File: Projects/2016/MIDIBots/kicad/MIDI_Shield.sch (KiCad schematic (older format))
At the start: 45 parts, among them IC1 PC900V, K1 SERVO_1, K2 SERVO_2, K3 SERVO_3, P1 MIDI_IN, P2 MIDI_THRU, P3 PWR_IN, P4 MIDI_IN, P5 MIDI_THRU, P6 D6_PWM, P7 MIDI_RX_EN, P8 STEPPER, P9 D12, Q1 F12N10L, Q2 F12N10L, SW1 RESET, SW2 DIPS_04, SW3 SELF_TEST, U1 74HC14

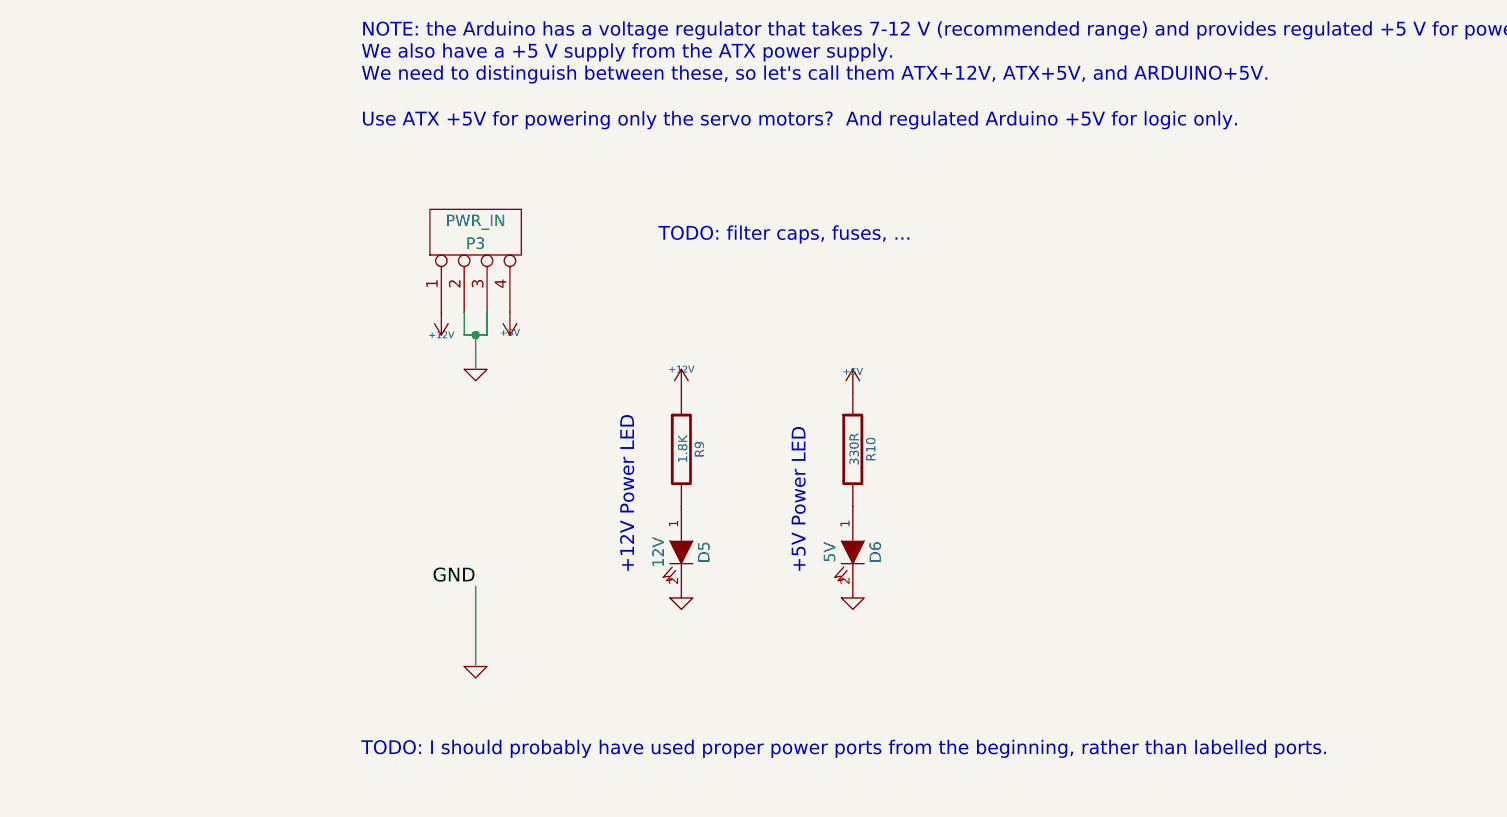
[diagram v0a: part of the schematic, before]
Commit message: Latest schematic and PCB design from work, plus extra libs we might need
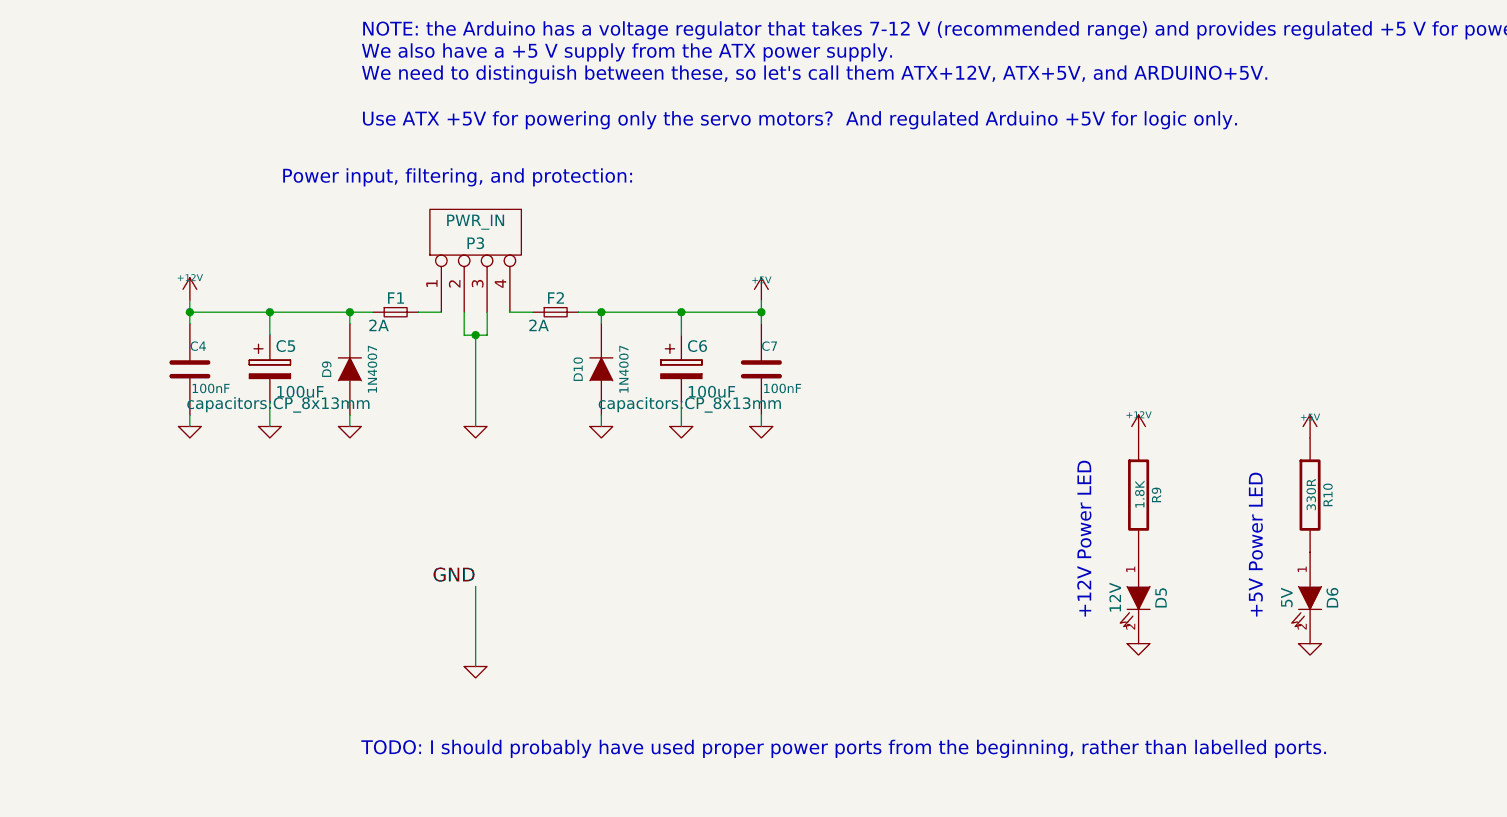
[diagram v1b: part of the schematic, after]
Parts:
- added C4, C7: 100nF, discret:C2, symbol C-RESCUE-MIDI_Shield
- added C5, C6: 100uF, capacitors:CP_8x13mm, symbol CP
- added D10, D9: 1N4007, discret:D4, symbol DIODE
- added F1, F2: 2A, discret:R7, symbol F_Small
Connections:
- net +12V: now also C4.1, C5.1, D9.2 (K), F1.1; no longer P3.1 (P1)
- net +5V: now also C6.1, C7.1, D10.2 (K), F2.2; no longer P3.4 (P4)
- net GND: now also C4.2, C5.2, C6.2, C7.2, D10.1 (A), D9.1 (A)
- new net: F1.2, P3.1 (P1)
- new net: F2.1, P3.4 (P4)
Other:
- note added: "Power input, filtering, and protection:"
- note removed: "TODO: filter caps, fuses, ..."
- moved on the sheet: D5, D6, R10, R9
